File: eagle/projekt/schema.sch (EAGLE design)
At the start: 21 parts, among them IC1 ESP12E_DEVKIT, IC2 LF50CP, J1 PSH02-02W, Q2 BC847CSMD

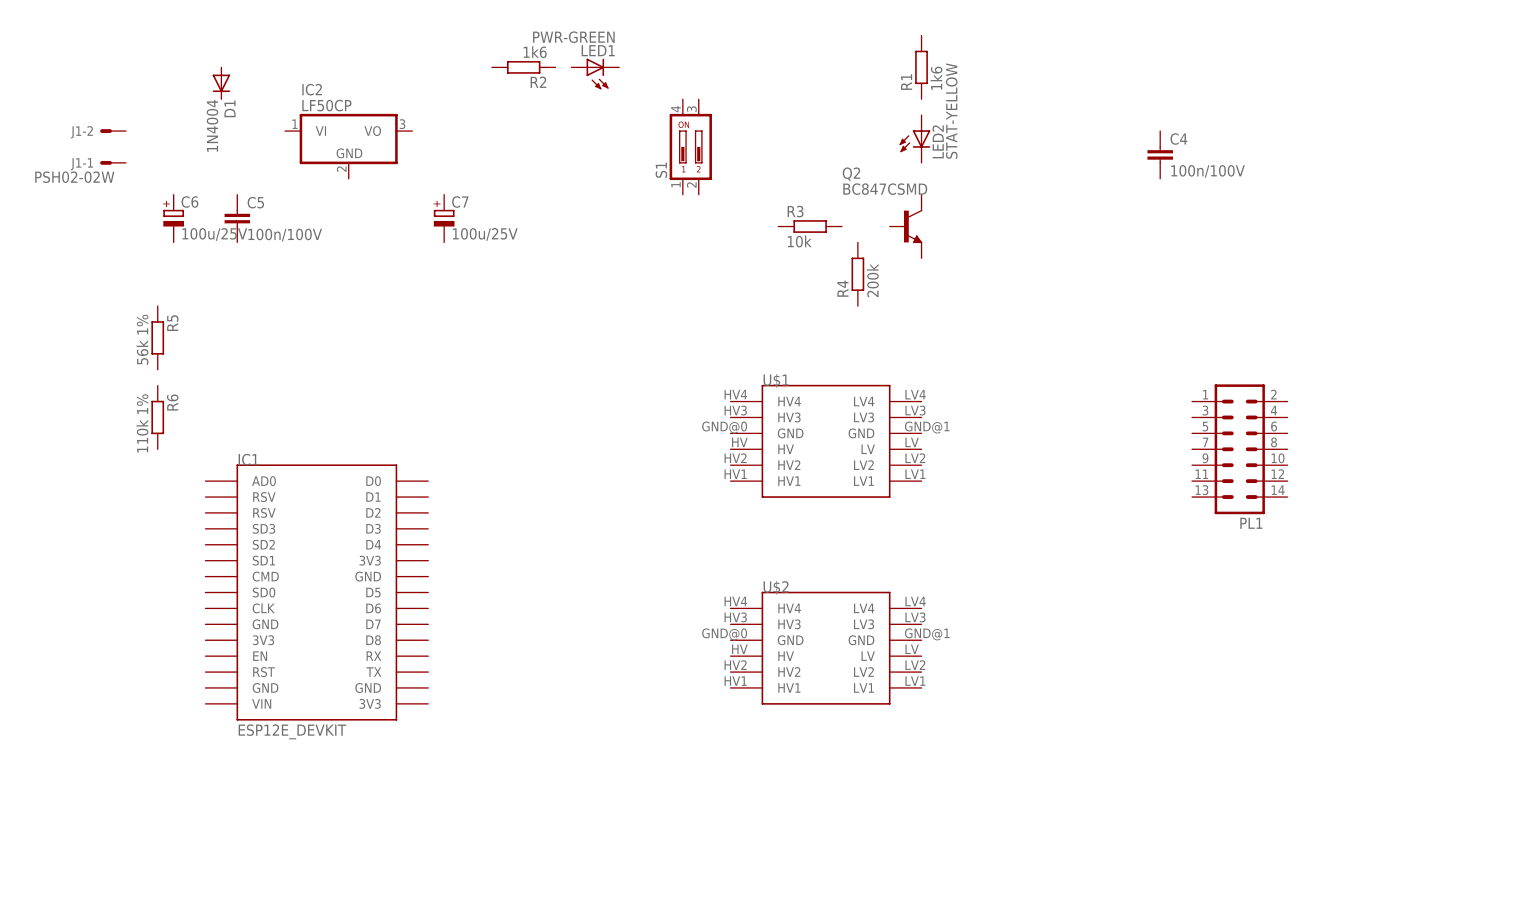
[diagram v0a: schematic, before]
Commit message: Schema
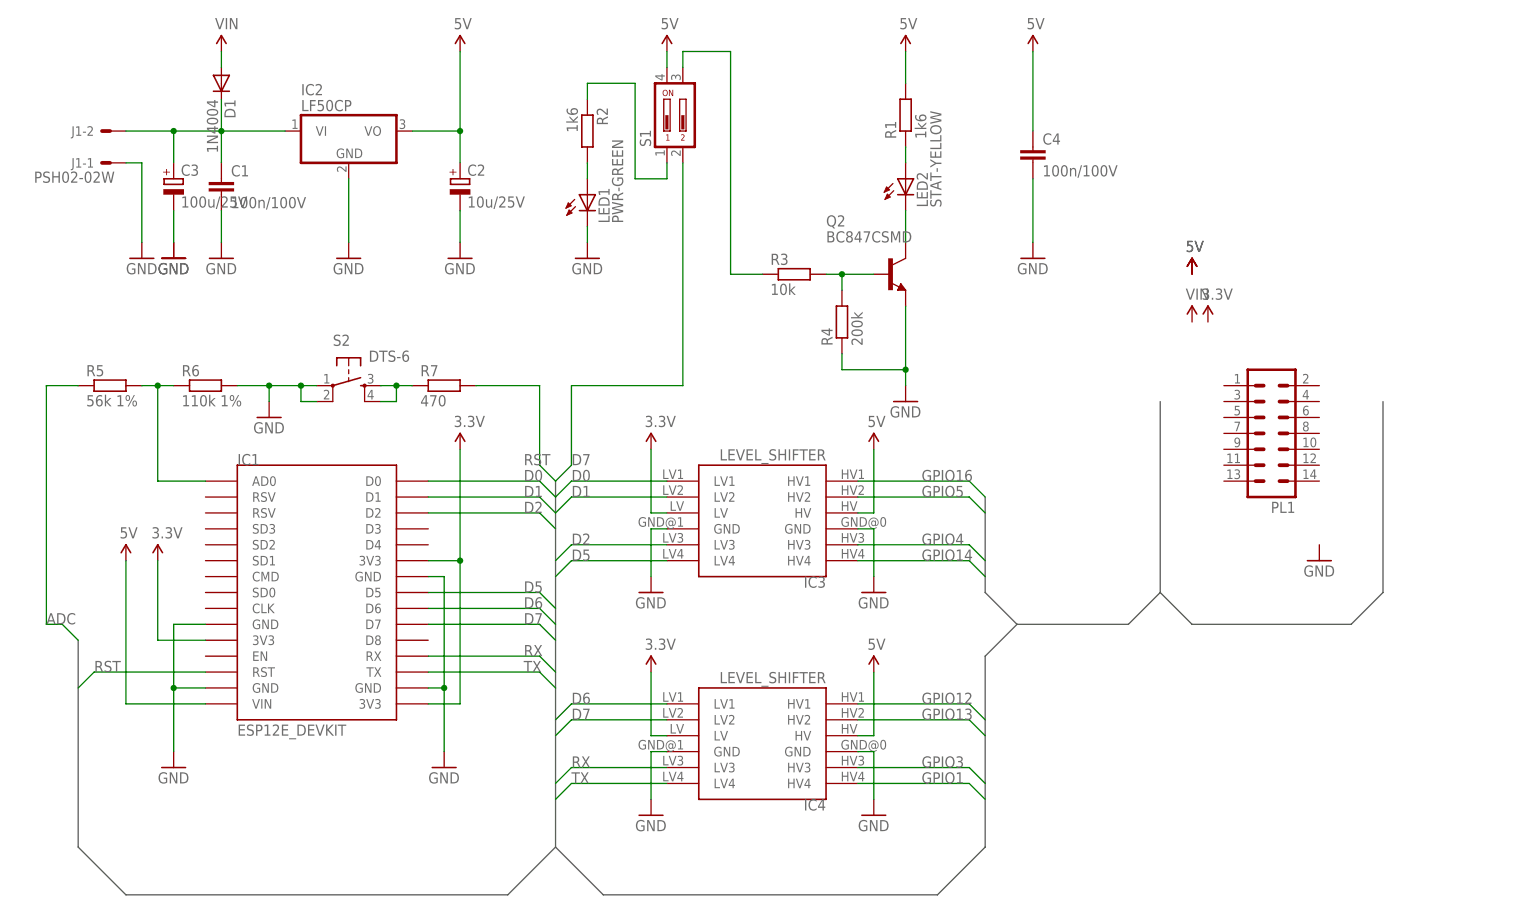
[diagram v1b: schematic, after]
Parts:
- removed C5: 100n/100V, parts_mix:C-EU025-025X050
- removed C6: 100u/25V, parts_mix:CPOL-EUE5-13
- removed C7: 100u/25V, parts_mix:CPOL-EUE3.5-8
- removed U$1, U$2: (no value), level_shifter:LEVEL_SHIFTER
- added C1: 100n/100V, parts:C-EUC025-025X050
- added C2: 10u/25V, parts:CPOL-EUE3,5-8
- added C3: 100u/25V, parts:CPOL-EUE5-13
- added IC3, IC4: LEVEL_SHIFTER, level_shifter:LEVEL_SHIFTER
- added R7: 470, rcl:R-EU_R1206
- added S2: DTS-6, switch-tact:DTS-6
- C4: device rcl:C-EU025-025X050 -> parts:C-EUC025-025X050
- IC2: device parts_mix:LF50CP -> parts:LF50CP
- PL1: device parts_mix:14V -> parts:14V
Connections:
- new net 3.3V: IC1.3V3@0, IC1.3V3@1, IC1.3V3@2, IC3.LV, IC4.LV
- new net 5V: C2.+, C4.1, IC1.VIN, IC2.VO, IC3.HV, IC4.HV, R1.2, S1.4
- new net ADC: R5.1
- new net D0: IC1.D0, IC3.LV1
- new net D1: IC1.D1, IC3.LV2
- new net D2: IC1.D2, IC3.LV3
- new net D5: IC1.D5, IC3.LV4
- new net D6: IC1.D6, IC4.LV1
- new net D7: IC1.D7, IC4.LV2, S1.2
- new net GND: C1.2, C2.-, C3.-, C4.2, IC1.GND@0, IC1.GND@1, IC1.GND@2, IC1.GND@3, IC2.GND, IC3.GND@0, IC3.GND@1, IC4.GND@0, IC4.GND@1, J1-1.S, LED1.C, Q2.E, R4.1, R6.2, S2.1, S2.2
- new net GPIO1: IC4.HV4
- new net GPIO12: IC4.HV1
- new net GPIO13: IC4.HV2
- new net GPIO14: IC3.HV4
- new net GPIO16: IC3.HV1
- new net GPIO3: IC4.HV3
- new net GPIO4: IC3.HV3
- new net GPIO5: IC3.HV2
- new net N$1: IC1.AD0, R5.2, R6.1
- new net N$14: C1.1, C3.+, D1.C, IC2.VI, J1-2.S
- new net N$2: LED1.A, R2.2
- new net N$3: R2.1, S1.1
- new net N$4: R7.1, S2.3, S2.4
- new net N$5: R3.1, S1.3
- new net N$6: Q2.B, R3.2, R4.2
- new net N$8: LED2.C, Q2.C
- new net N$9: LED2.A, R1.1
- new net RST: IC1.RST, R7.2
- new net RX: IC1.RX, IC4.LV3
- new net TX: IC1.TX, IC4.LV4
- new net VIN: D1.A
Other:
- moved on the sheet: C4, LED1, LED2, PL1, Q2, R1, R2, R3, R4, R5, R6, S1

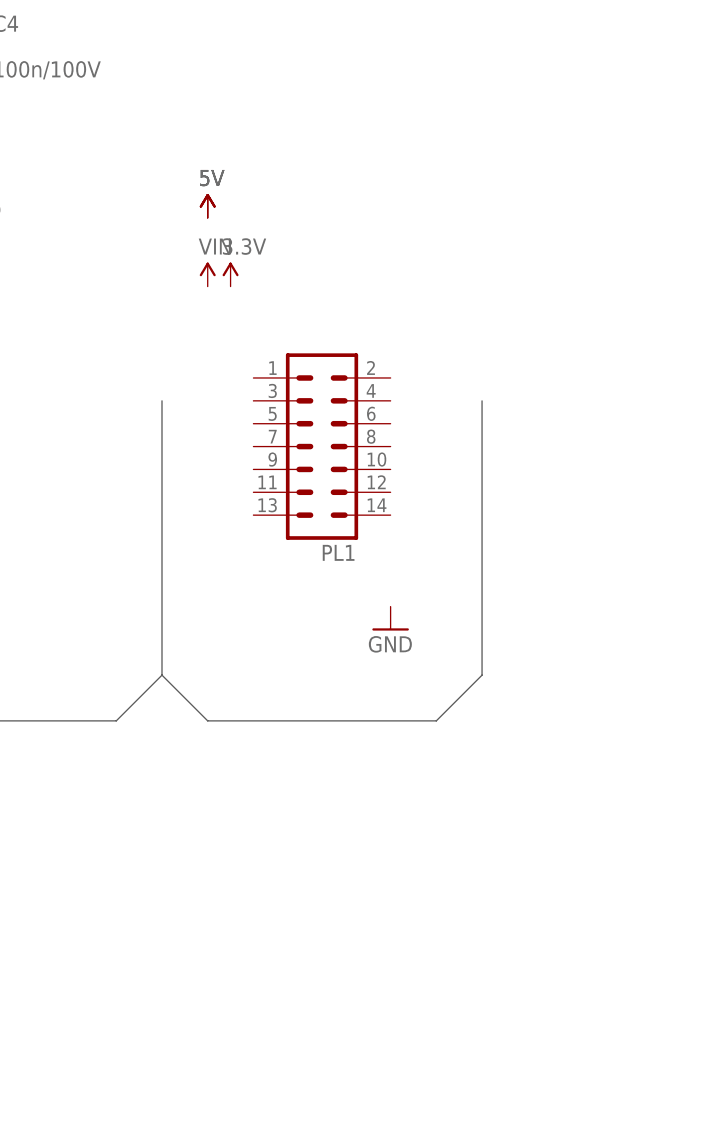
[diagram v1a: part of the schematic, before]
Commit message: Schema
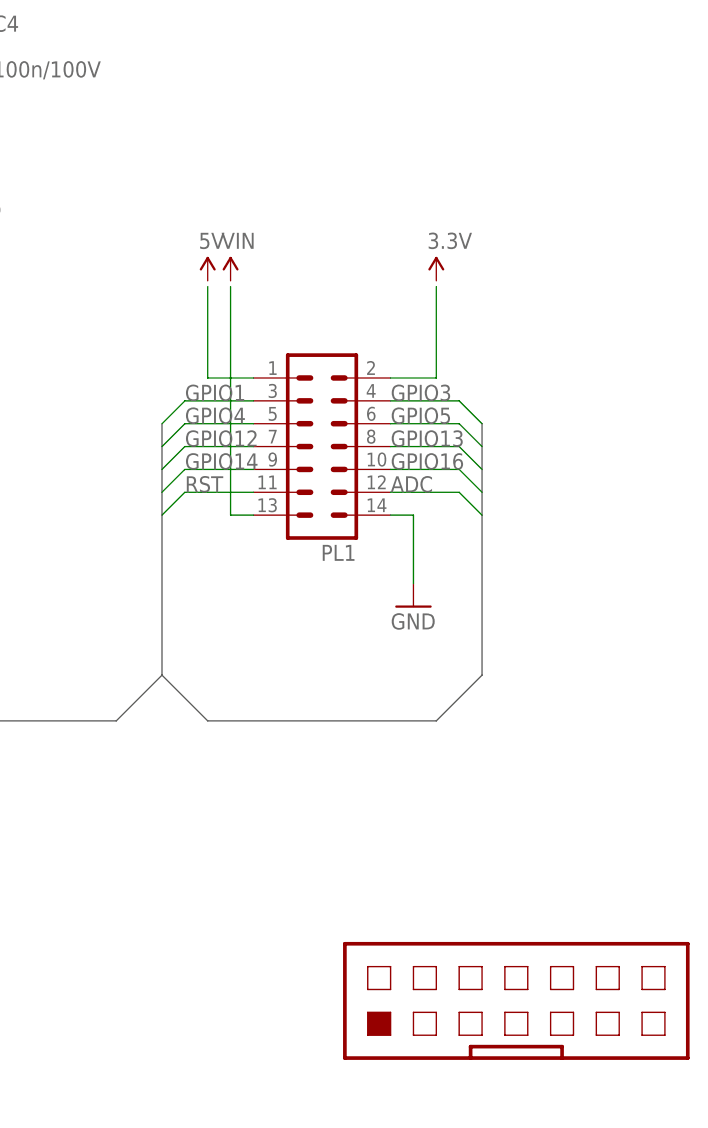
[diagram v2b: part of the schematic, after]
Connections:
- new net N$10: PL1.13
- new net N$11: PL1.2
- new net N$7: PL1.1
- net ADC: now also PL1.12
- net GND: now also PL1.14
- net GPIO1: now also PL1.3
- net GPIO12: now also PL1.7
- net GPIO13: now also PL1.8
- net GPIO14: now also PL1.9
- net GPIO16: now also PL1.10
- net GPIO3: now also PL1.4
- net GPIO4: now also PL1.5
- net GPIO5: now also PL1.6
- net RST: now also PL1.11
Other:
- note added: "+3.3V"
- note added: "+5V"
- note added: "1"
- note added: "14"
- note added: "2"
- note added: "ADC"
- note added: "GND"
- note added: "GPIO1/TX"
- note added: "GPIO12"
- note added: "GPIO13"
- note added: "GPIO14"
- note added: "GPIO16"
- note added: "GPIO3/RX"
- note added: "GPIO4"
- note added: "GPIO5"
- note added: "RST"
- note added: "VIN"
